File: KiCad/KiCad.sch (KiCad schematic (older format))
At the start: 18 parts, among them J1 HV input, U1 PQMC3-D12-S12-S, U2 LM311N_NOPB

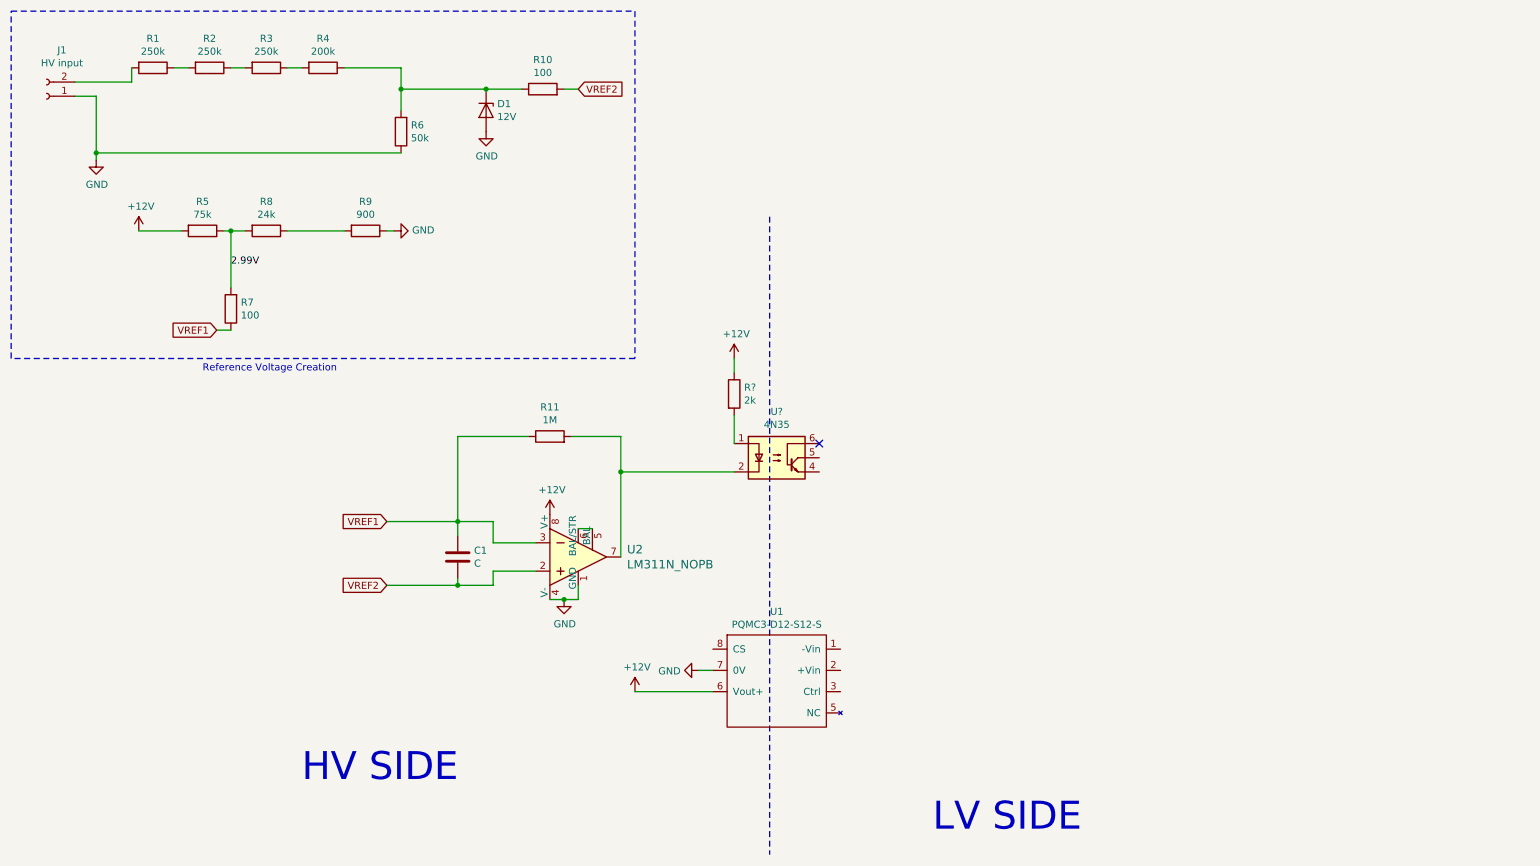
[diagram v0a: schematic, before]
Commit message: Schematic Complete
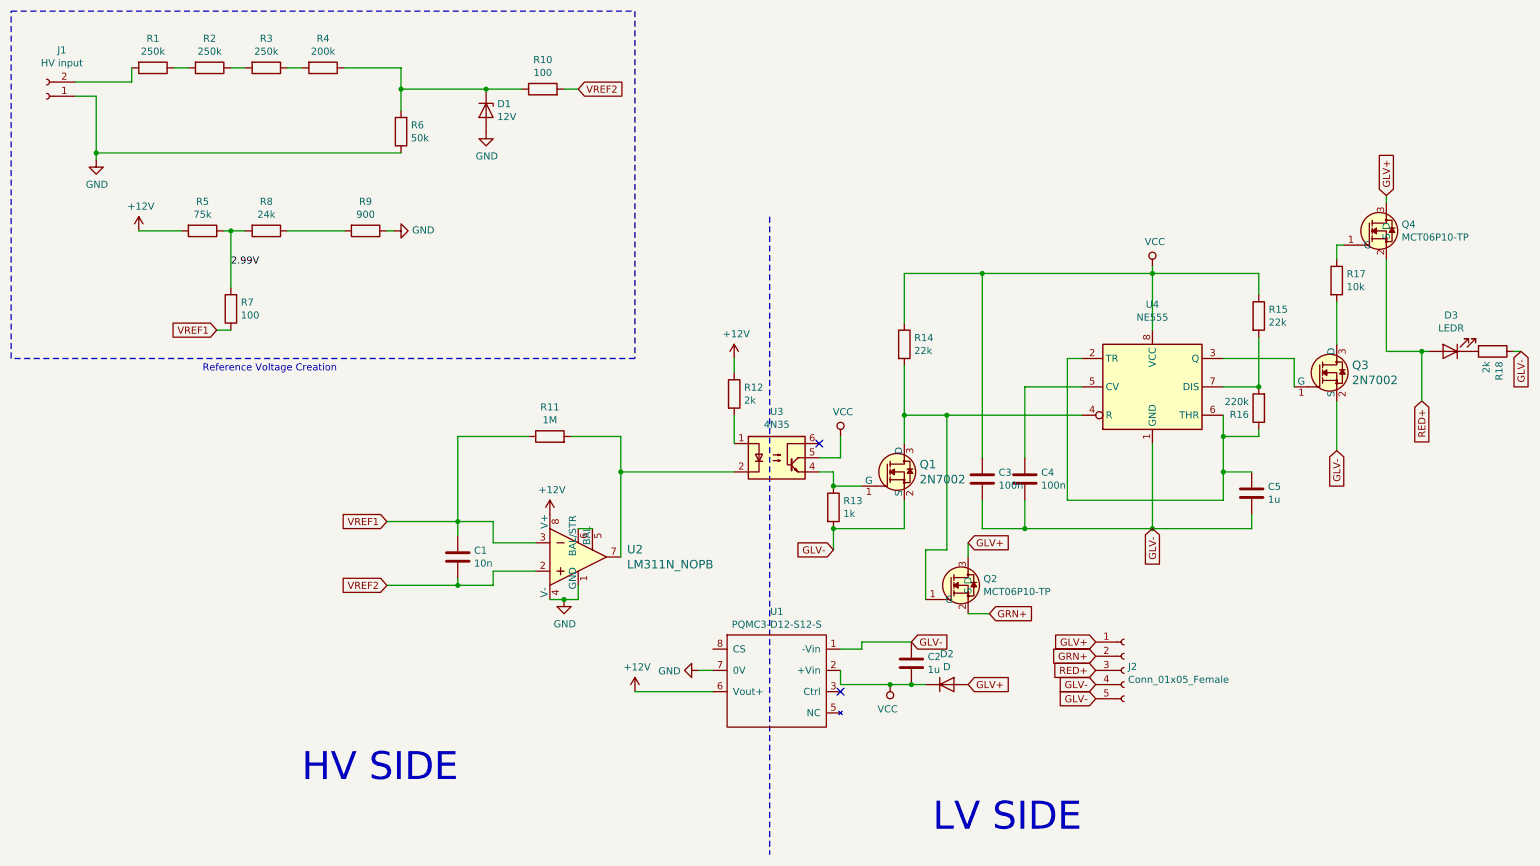
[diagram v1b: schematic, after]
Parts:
- added C2, C5: 1u, symbol Device:C
- added C3, C4: 100n, symbol Device:C
- added D2: D, symbol Device:D
- added D3: LEDR, symbol Device:LED
- added J2: Conn_01x05_Female, symbol Connector:Conn_01x05_Female
- added Q1, Q3: 2N7002, digikey-footprints:SOT-23-3, symbol dk_Transistors-FETs-MOSFETs-Single:2N7002
- added Q2, Q4: MCT06P10-TP, symbol Lukas_Library:MCT06P10-TP
- added R13: 1k, symbol Device:R
- added R14, R15: 22k, symbol Device:R
- added R16: 220k, symbol Device:R
- added R17: 10k, symbol Device:R
- added R18: 2k, symbol Device:R
- added U4: NE555, symbol Timer:NE555
- C1: value C -> 10n
- gave numbers to parts that had none: 2
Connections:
- net GLV-: now reaches U1.1 (-Vin)
- net GLV-: now also C2.1, C3.2, C4.2, C5.2, J2.4 (Pin_4), J2.5 (Pin_5), Q1.2 (S), Q3.2 (S), R13.2, R18.1, U4.1 (GND)
- net VCC: now reaches U1.2 (+Vin)
- net VCC: now also U3.5, C2.2, C3.1, D2.1 (K), R14.1, R15.1, U4.8 (VCC)
- net at U3.4: now also Q1.1 (G), R13.1
- new net: C5.1, R16.1, U4.2 (TR), U4.6 (THR)
- new net: Q3.1 (G), U4.3 (Q)
- new net: Q1.3 (D), Q2.1 (G), R14.2, U4.4 (R)
- new net: C4.1, U4.5 (CV)
- new net: R15.2, R16.2, U4.7 (DIS)
- new net: Q3.3 (D), R17.2
- new net: Q4.1 (G), R17.1
- new net: D3.1 (K), R18.2
- new net GLV+: D2.2 (A), J2.1 (Pin_1), Q2.3 (D), Q4.3 (D)
- new net GRN+: J2.2 (Pin_2), Q2.2 (S)
- new net RED+: D3.2 (A), J2.3 (Pin_3), Q4.2 (S)
- no-connect marks 1 -> 2
